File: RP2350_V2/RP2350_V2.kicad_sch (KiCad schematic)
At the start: 114 parts, among them IC1 DMP1045U-7, IC2 DMP1045U-7, IC3 DMP1045U-7, IC4 DMP1045U-7, IC5 DMP1045U-7, IC6 DMP1045U-7, J1 Conn_01x04_Pin, J10 S0991-46R, J2 S0991-46R, J3 USB_C_Receptacle_USB2.0_16P, J5 Conn_01x08_Socket, J6 Conn_01x02_Pin, J7 Conn_01x04_Pin, J8 S0991-46R, J9 S0991-46R, SW1 PTS 647 SN50 SMTR2 LFS, SW10 PTS 647 SN50 SMTR2 LFS, SW11 PTS 647 SN50 SMTR2 LFS, SW12 PTS 647 SN50 SMTR2 LFS, SW13 PTS 647 SN50 SMTR2 LFS, SW14 PTS 647 SN50 SMTR2 LFS, SW4 PTS 647 SN50 SMTR2 LFS, SW9 PTS 647 SN50 SMTR2 LFS, U1 RP2350_60QFN, U2 W25Q128JVS, U3 TPS62811QWRWYRQ1, U4 MCP73812T-420I-OT, U5 TLV3012AIDCKR, U6 74HC14, X1 ABM8-272-T3

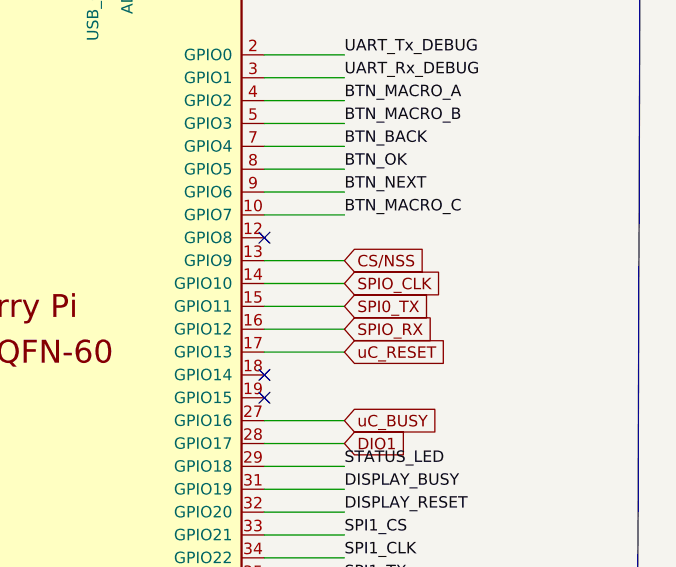
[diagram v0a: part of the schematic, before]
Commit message: dfdjfjh pt2
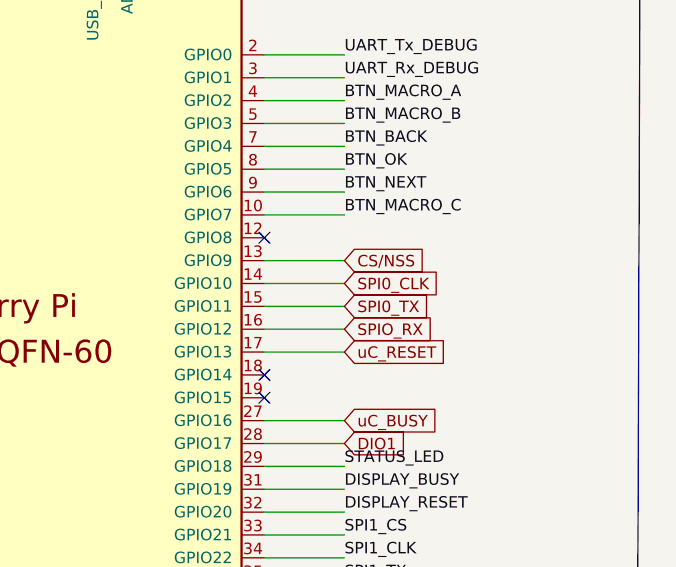
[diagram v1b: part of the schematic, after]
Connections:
- net SPIO_CLK is gone; now on net SPI0_CLK: U1.14 (GPIO10)
